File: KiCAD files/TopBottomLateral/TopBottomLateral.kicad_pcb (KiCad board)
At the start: 2 copper layers, 69.9 x 107.3 mm, 10 parts

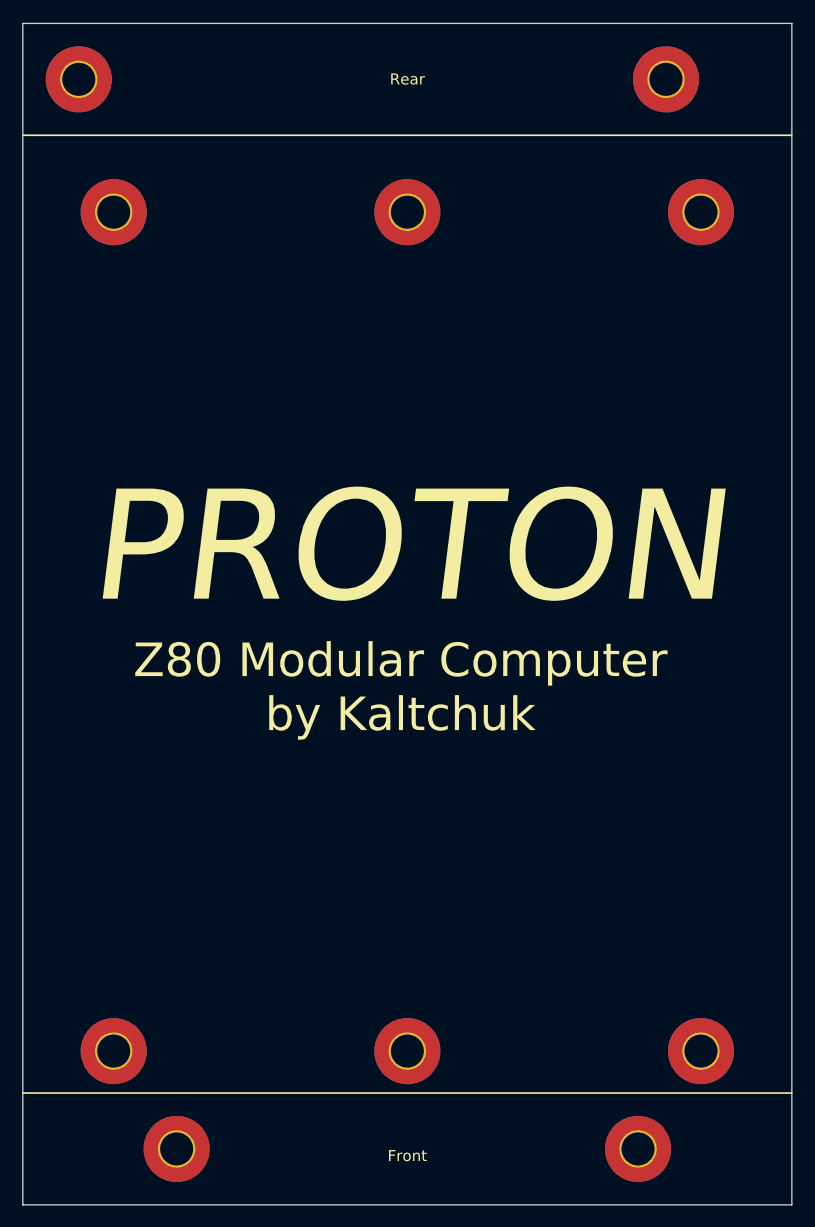
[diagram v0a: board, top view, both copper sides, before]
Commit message: PCBs
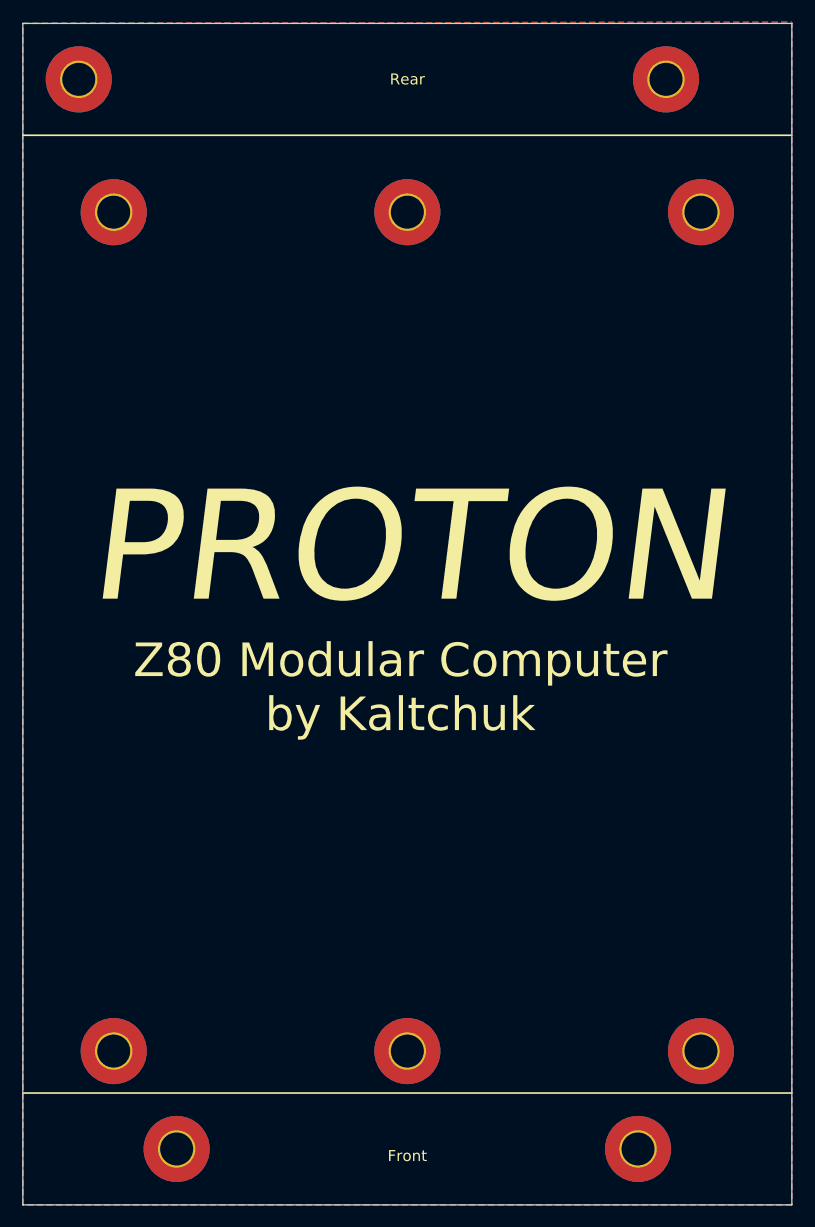
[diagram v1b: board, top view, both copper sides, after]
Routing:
- added copper zone on B.Cu, net (none)
- added copper zone on F.Cu, net (none)
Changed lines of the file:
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@@
     (pad_to_mask_clearance 0)
     (pcbplotparams
-      (layerselection 0x00010fc_ffffffff)
+      (layerselection 0x00010f0_ffffffff)
       (disableapertmacros false)
       (usegerberextensions false)
@@
       (outputformat 1)
       (mirror false)
-      (drillshape 1)
+      (drillshape 0)
       (scaleselection 1)
       (outputdirectory "")
@@
     (effects (font (size 1 1) (thickness 0.15)))
   )
+  (zone (net 0) (net_name "") (layers F&B.Cu) (hatch edge 0.508)
+    (connect_pads (clearance 0.508))
+    (min_thickness 0.254) (filled_areas_thickness no)
+    (fill yes (thermal_gap 0.508) (thermal_bridge_width 0.508))
+    (polygon
+      (pts
+        (xy 128.27 144.145)
+        (xy 58.42 144.145)
+        (xy 58.42 36.83)
+        (xy 128.27 36.703)
+      )
+    )
+  )
 )
